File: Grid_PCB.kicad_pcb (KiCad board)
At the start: 2 copper layers, 223.2 x 22 mm, 44 parts, among them J1 Conn_01x04_Female, J10 LED_Conn, J11 Power_Conn, J2 Conn_01x04_Female, J3 Conn_01x04_Female, J4 Conn_01x04_Female, J5 Conn_01x04_Female, J6 Conn_01x04_Female, J7 Conn_01x04_Female, J8 Conn_01x04_Female, J9 ESP_Conn, U1 SN74HC151N

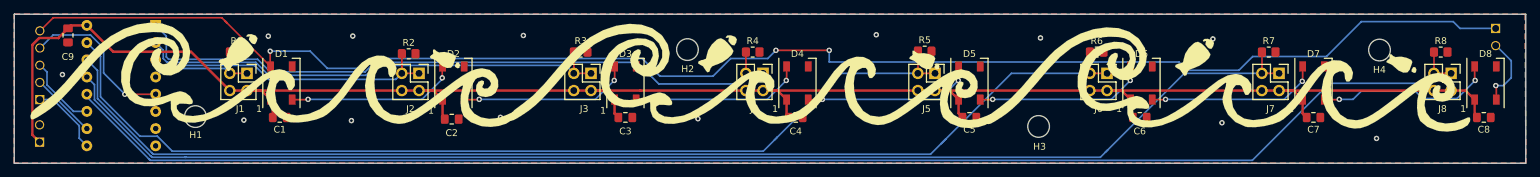
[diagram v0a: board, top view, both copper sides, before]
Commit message: wave fish thin, like this one the best
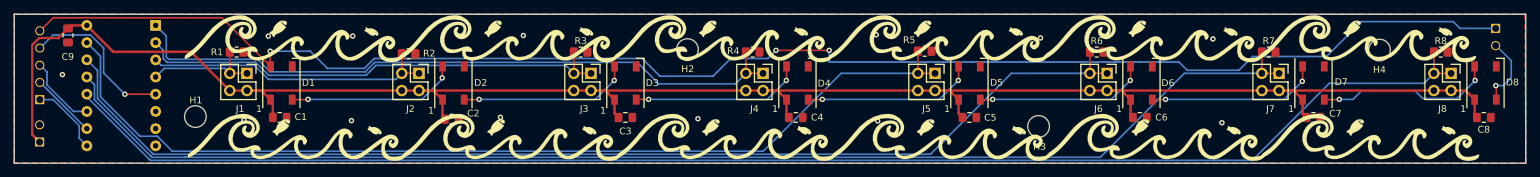
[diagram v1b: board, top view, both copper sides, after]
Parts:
- removed the G*** at (223.4, 92.2)
- removed the G*** at (153.0, 91.7)
- removed the G*** at (82.2, 91.5)
- added G***: LOGO, grid:wave_fish_small, F.Cu at (243.3, 86.9)
- added G***: LOGO, grid:wave_fish_small, F.Cu at (148.7, 101.5)
- added G***: LOGO, grid:wave_fish_small, F.Cu at (116.9, 101.5)
- added G***: LOGO, grid:wave_fish_small, F.Cu at (85.2, 101.5)
- added G***: LOGO, grid:wave_fish_small, F.Cu at (148.2, 86.9)
- added G***: LOGO, grid:wave_fish_small, F.Cu at (211.6, 86.9)
- added G***: LOGO, grid:wave_fish_small, F.Cu at (84.8, 86.9)
- added G***: LOGO, grid:wave_fish_small, F.Cu at (179.9, 86.9)
- added G***: LOGO, grid:wave_fish_small, F.Cu at (116.5, 86.9)
- added G***: LOGO, grid:wave_fish_small, F.Cu at (243.8, 101.5)
- added G***: LOGO, grid:wave_fish_small, F.Cu at (212.1, 101.5)
- added G***: LOGO, grid:wave_fish_small, F.Cu at (180.4, 101.5)
